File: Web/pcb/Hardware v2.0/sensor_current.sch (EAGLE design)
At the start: 7 parts, among them J1 22-27-2031-03, U1 MLX91208LDC-CAL-000-TU

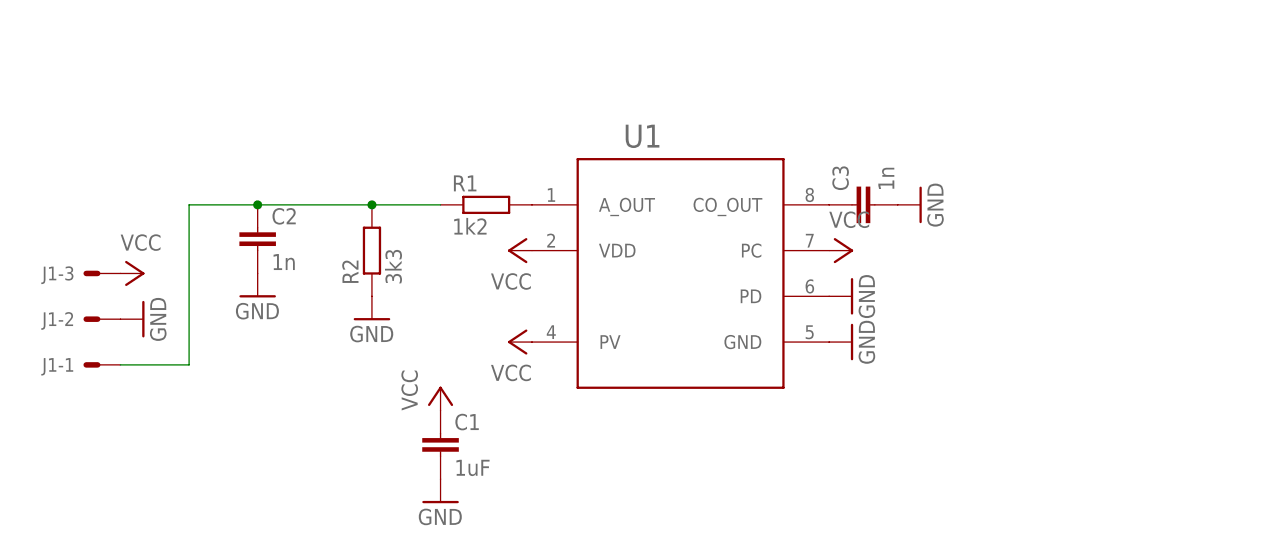
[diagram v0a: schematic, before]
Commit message: updates
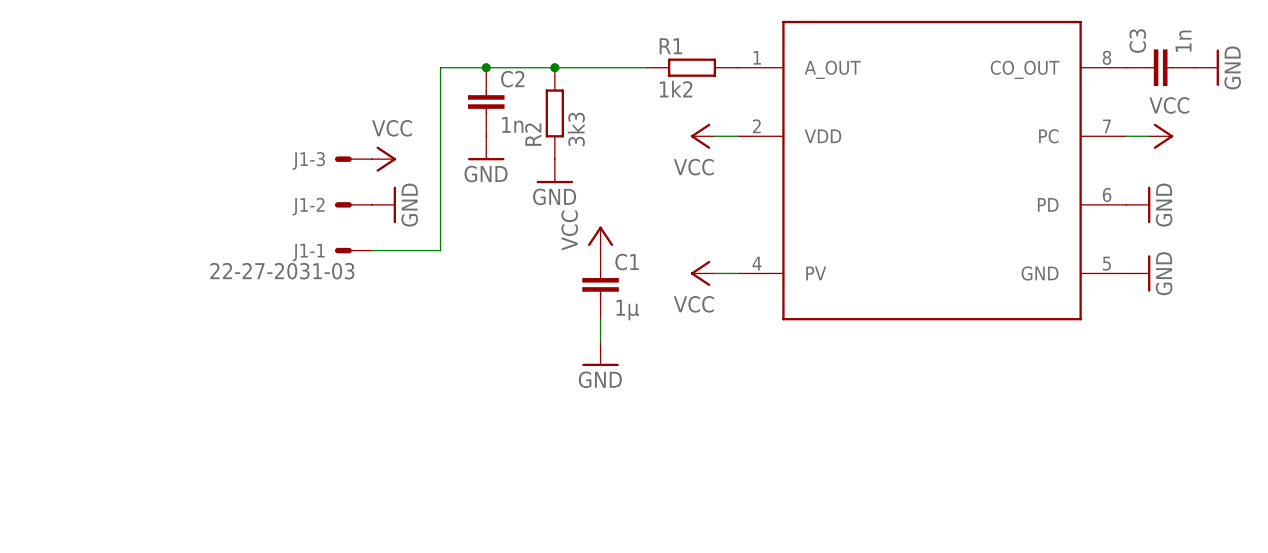
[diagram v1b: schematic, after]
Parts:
- removed U1: MLX91208LDC-CAL-000-TU, MLX91208:MLX91208LDC-CAL-000-TU
- added IC1: MLX91205, melexis:MLX91205
- C1: value 1uF -> 1µ
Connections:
- removed net N$3 (its old number): R1.2, U1.A_OUT
- new net N$2: C3.1, IC1.CO_OUT
- net GND: now also IC1.GND, IC1.PD; no longer U1.GND, U1.PD
- net N$1: now also IC1.A_OUT, R1.2; no longer C3.1, U1.CO_OUT
- net VCC: now also IC1.PC, IC1.PV, IC1.VDD; no longer U1.PC, U1.PV, U1.VDD
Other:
- moved on the sheet: C1, C2, C3, J1-1, J1-2, J1-3, R1, R2
